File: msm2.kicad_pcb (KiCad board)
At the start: 2 copper layers, 150 x 100 mm, 69 parts, among them J1 PowerH, J10 Conn_01x36, J11 Conn_01x36, J12 Conn_01x36, J2 PowerL, J3 USB_vcc, J4 Conn_ARM_JTAG_SWD_20, J5 usb_new, J6 JUMP_usb, J7 JUMP_vdd, J8 JUMP_gnd, J9 Conn_01x36, SW1 SW_Push, SW2 SW_Push1, SW3 SW_Push2, SW4 SW_Push3, SW5 SW_Push, U1 STM32F407ZETx, U2 AMS1117-3.3, U3 CH340C, Y1 25M, Y2 32.768k

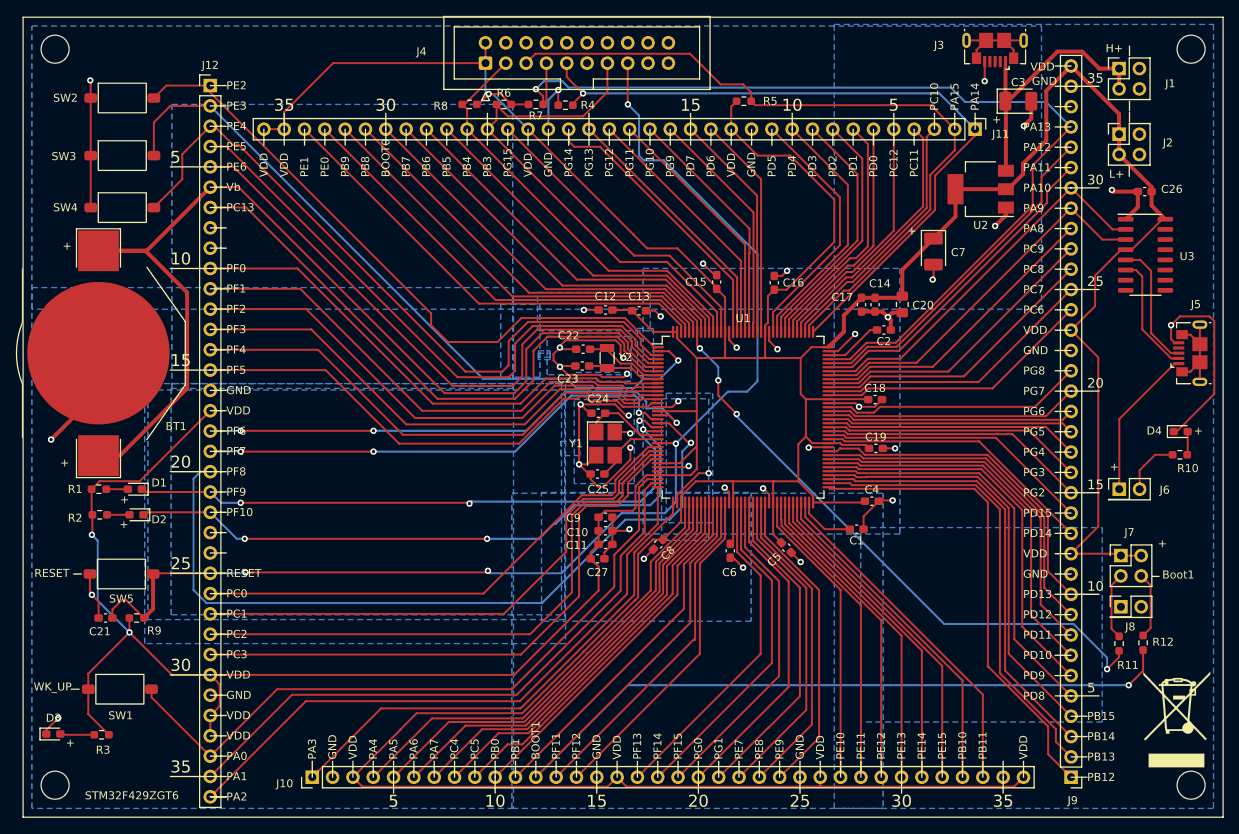
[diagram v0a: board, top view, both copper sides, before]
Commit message: pcb v3.0
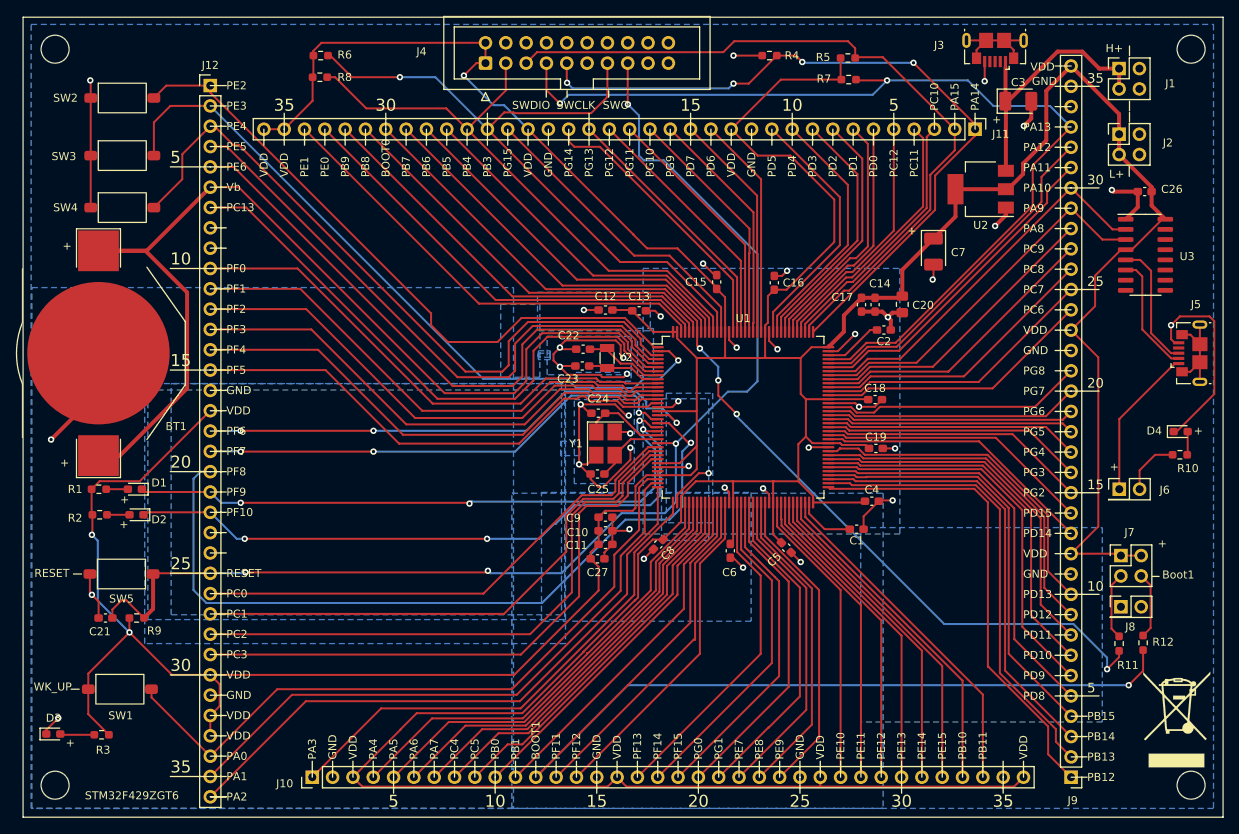
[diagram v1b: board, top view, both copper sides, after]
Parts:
- moved R7 39.2 mm to (103.2, 7.80)
- moved R4 26.2 mm to (93.3, 4.80)
- moved R6 23.7 mm to (37.2, 4.80), turned to 180 degrees
- moved R8 19.0 mm to (37.1, 7.50), turned to 180 degrees
- moved R5 14.1 mm to (103.1, 5.10)
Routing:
- net /PB3: track 63.6 -> 85.4 mm, vias 0 -> 1
- net /PB4: track 53.3 -> 72.8 mm
- net VDD: track 710.6 -> 725.1 mm
- net GND: track 218.4 -> 214.7 mm
- net /PA14: track 91.2 -> 93.4 mm, vias 1 -> 4
- net /PA15: track 91.9 -> 93.3 mm
- net /PA13: track 122.6 -> 122.5 mm, vias 1 -> 2
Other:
- board text added: "SWCLK"
- board text added: "SWDIO"
- board text added: "SWO"
